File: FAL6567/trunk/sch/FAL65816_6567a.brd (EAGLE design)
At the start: 100 x 80 mm, 34 parts, among them IC1 74LVC04D, IC10 74LVC245DW, IC12 74LVC00D, IC13 74LVC138D, IC2 74LVC245DW, IC4 74LVC573, IC5 74LVC573, IC7 74LVC573, Q1 2N2222, U1 65C22

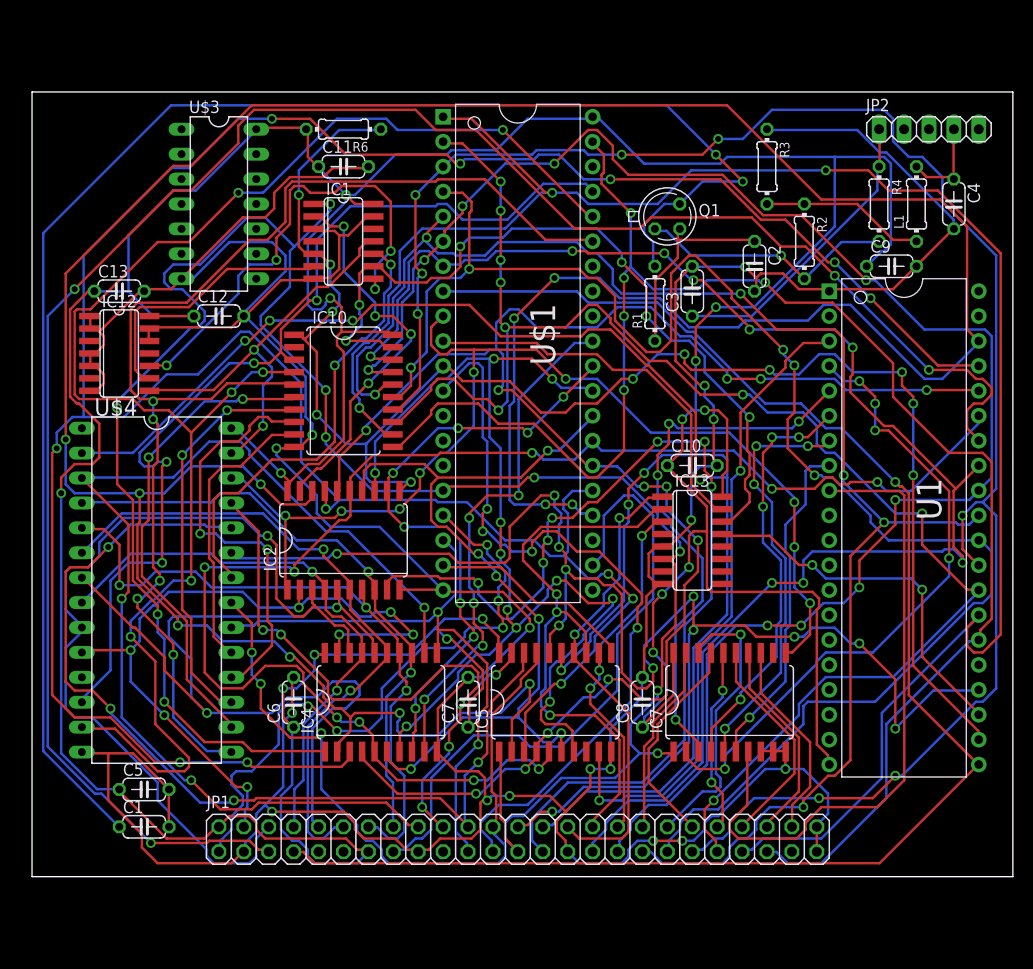
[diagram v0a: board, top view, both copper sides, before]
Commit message: FAL65816 - update
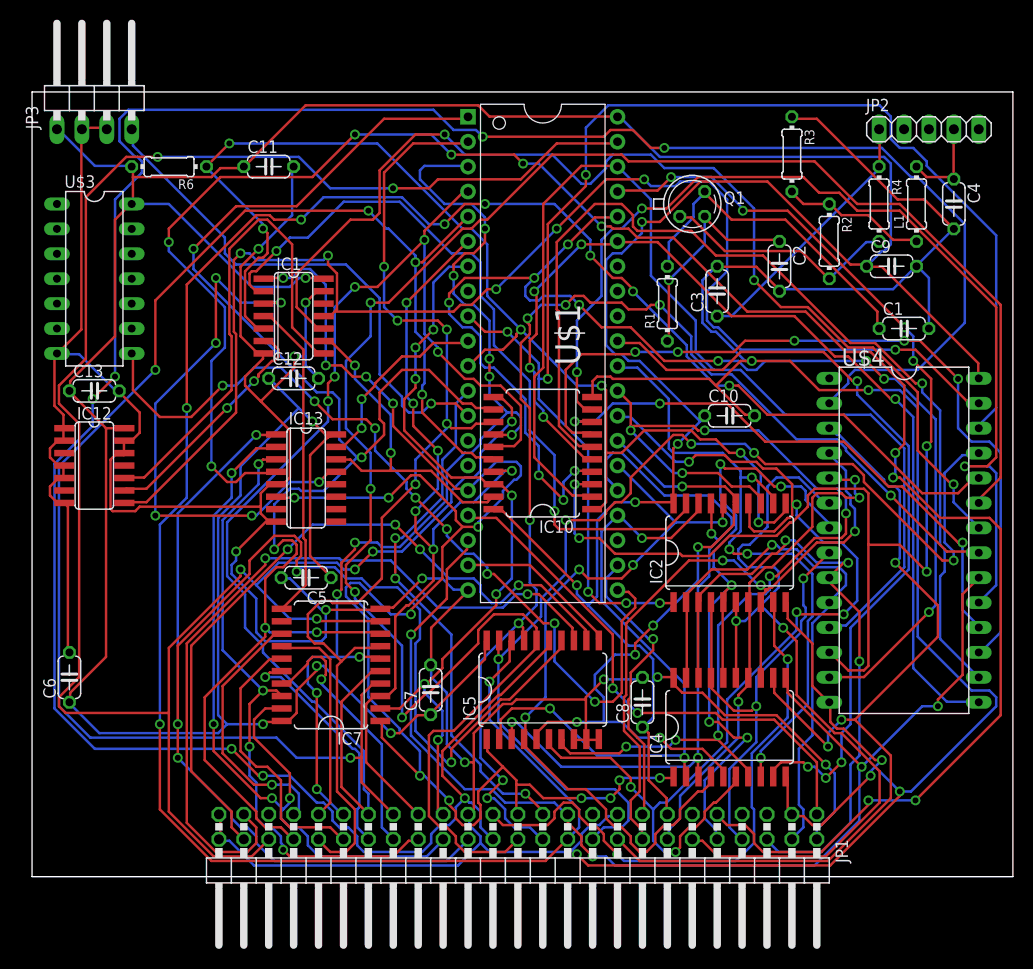
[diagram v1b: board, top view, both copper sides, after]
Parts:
- removed U1: 65C22, 65xxx:DIP-40
- added JP3: (no value), pinhead:1X04/90
- JP1: device pinhead:2X25 -> pinhead:2X25/90
- moved C1 92.6 mm to (88.9, 55.9)
- moved U$4 76.4 mm to (88.9, 34.3)
- moved IC7 40.8 mm to (30.5, 21.6), turned to 90 degrees
- moved IC13 39.9 mm to (27.9, 40.6)
- moved IC2 39.4 mm to (71.1, 33.0)
- moved IC4 35.7 mm to (71.1, 15.2)
- moved C5 27.2 mm to (27.9, 30.5), turned to 180 degrees
- moved C6 23.0 mm to (3.81, 20.3)
- moved IC10 21.3 mm to (52.1, 43.2), turned to 90 degrees
- moved R6 18.2 mm to (14.0, 72.4)
- moved U$3 14.8 mm to (6.35, 61.0)
- moved IC12 11.7 mm to (6.35, 41.9)
- moved C13 10.5 mm to (6.35, 49.5)
- moved C12 9.92 mm to (26.7, 50.8)
- moved IC1 9.16 mm to (26.7, 57.1)
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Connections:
- removed net C6522N: IC13.13, U1.23
- removed net PA0: IC5.8, U1.2
- removed net PA1: IC5.9, U1.3
- removed net PA2: IC7.2, U1.4
- removed net PA3: IC7.3, U1.5
- removed net PA4: IC7.4, U1.6
- removed net PA5: IC7.5, U1.7
- removed net PA6: IC7.6, U1.8
- removed net PA7: IC7.7, U1.9
- new net CSAH: IC1.4, IC7.11
- new net CSAHN: IC1.3, IC13.13
- net +12V: now also JP3.4
- net A11: no longer U1.24
- net A14: now also IC7.19; no longer IC5.13
- net A15: now also IC7.18; no longer IC5.12
- net A16: now also IC7.17; no longer IC7.19
- net A17: now also IC7.16; no longer IC7.18
- net A18: now also IC7.15; no longer IC7.17
- net A19: now also IC7.14; no longer IC7.16
- net A20: now also IC7.13; no longer IC7.15
- net A21: now also IC7.12; no longer IC7.14
- net A22: now also IC5.13; no longer IC7.13
- net A23: now also IC5.12; no longer IC7.12
- net D0: now also IC7.2; no longer U1.33
- net D1: now also IC7.3; no longer U1.32
- net D2: now also IC7.4; no longer U1.31
- net D3: now also IC7.5; no longer U1.30
- net D4: now also IC7.6; no longer U1.29
- net D5: now also IC7.7; no longer U1.28
- net D6: now also IC7.8; no longer U1.27
- net D7: now also IC7.9; no longer U1.26
- net GND: now also IC5.8, IC5.9, JP3.2, JP3.3; no longer IC1.3, IC7.8, IC7.9, U1.1
- net IRQN: no longer U1.21
- net PH2: no longer U1.25
- net PU1: no longer IC7.11
- net RESN: no longer U1.34
- net RWB: no longer U1.22
- net VA0: no longer U1.38
- net VA1: no longer U1.37
- net VA2: no longer U1.36
- net VA3: no longer U1.35
- net VCC: now also JP3.1; no longer U1.20
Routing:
- net VA0: track 324.1 -> 65.2 mm, vias 11 -> 3
- net VA1: track 299.2 -> 74.3 mm, vias 12 -> 3
- net IOSELN: track 0.00 -> 203.5 mm, vias 0 -> 10
- net RESN: track 197.2 -> 0.00 mm, vias 4 -> 0
- net IRQN: track 161.1 -> 0.00 mm, vias 1 -> 0
- net A9: track 98.4 -> 226.3 mm, vias 4 -> 9
- net VVID: track 160.3 -> 33.8 mm, vias 2 -> 0
- net D8: track 0.00 -> 112.9 mm
- net A13: track 48.5 -> 153.1 mm, vias 2 -> 5
- net GND: track 457.7 -> 559.2 mm, vias 16 -> 14
- net WCLRN: track 42.8 -> 140.0 mm, vias 2 -> 6
- net VA2: track 172.7 -> 77.2 mm, vias 12 -> 4
- net A12: track 168.8 -> 264.2 mm
- net CCLK: track 0.00 -> 88.5 mm, vias 0 -> 8
- net D1: track 169.1 -> 84.5 mm, vias 9 -> 6
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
